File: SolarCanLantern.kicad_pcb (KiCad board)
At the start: 2 copper layers, 30.5 x 19 mm, 15 parts, among them Q1 2N7002, Q2 2N7002, SW1 SW_Push, U1 ATTINY13-20SSU, U2 MAX40200

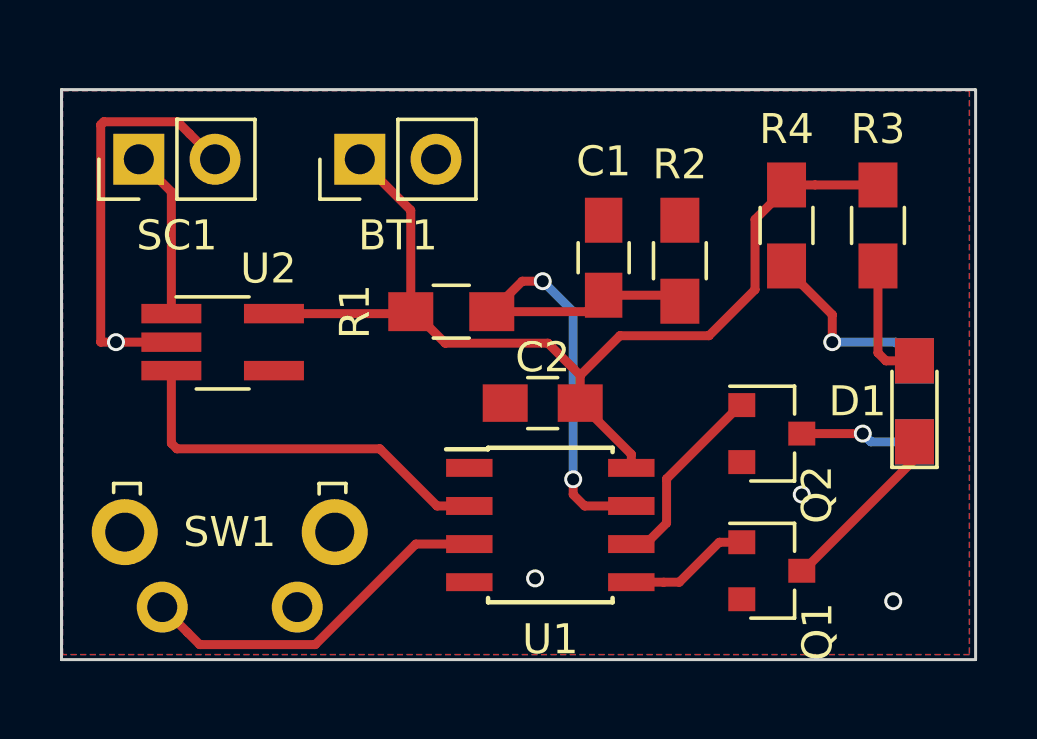
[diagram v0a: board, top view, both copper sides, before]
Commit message: slightly reorganize board
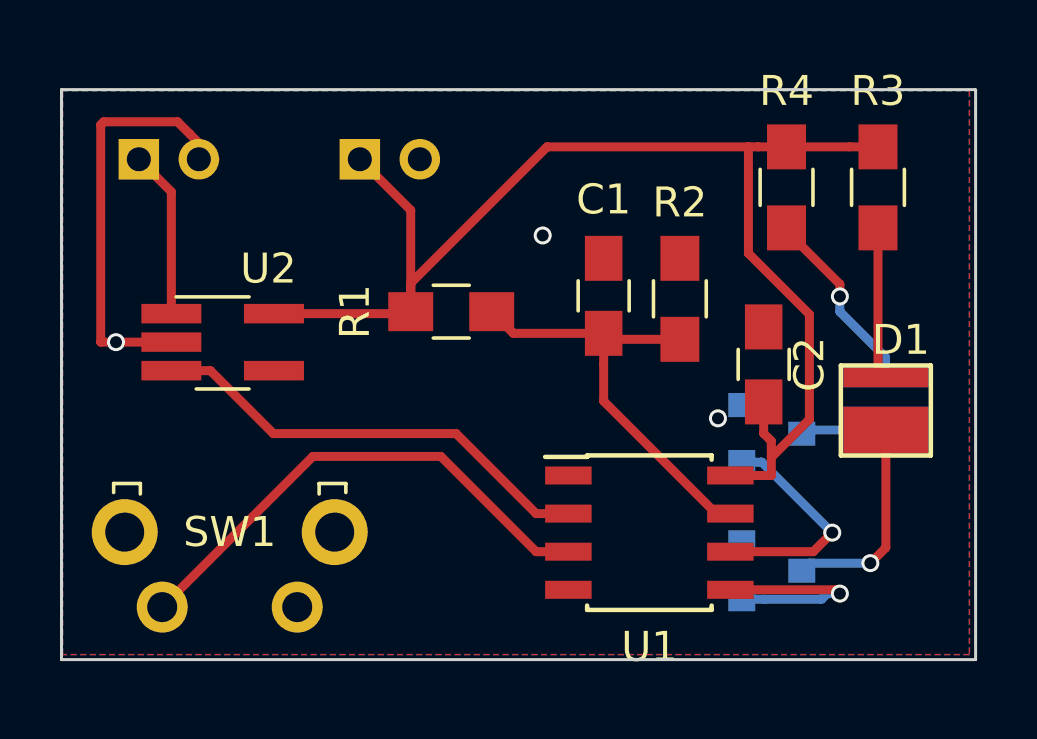
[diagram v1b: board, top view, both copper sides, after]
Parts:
- BT1, SC1: footprint Socket_Strips:Socket_Strip_Straight_1x02_Pitch2.54mm -> Socket_Strips:Socket_Strip_Straight_1x02_Pitch2.00mm; moved to B.Cu
- D1, D2: footprint LEDs:LED_0805_HandSoldering -> Footprints:CreeXLampXH-G
- Q1, Q2: moved to B.Cu
- moved C2 7.48 mm to (220.5, 87.1), turned to 90 degrees
- moved U1 3.31 mm to (216.7, 92.7)
- moved D2 1.48 mm to (224.0, 88.1)
- moved C1 1.27 mm to (215.1, 84.8)
- moved R2 1.27 mm to (217.7, 84.9)
- moved R3 1.27 mm to (224.3, 81.2)
- moved R4 1.27 mm to (221.2, 81.2)
- moved D1 0.49 mm to (225.0, 88.1)
- turned BT1 to 270 degrees
- turned SC1 to 270 degrees
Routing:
- net +BATT: track 34.7 -> 44.6 mm
- net /Switch: track 12.1 -> 16.9 mm
- net /VBatt_Divider: track 18.3 -> 14.7 mm, vias 2 -> 0
- net /LEDA: track 4.23 -> 7.05 mm, vias 0 -> 1
- net /~SOLAR: track 13.2 -> 15.2 mm
- net /LEDB: track 6.47 -> 7.65 mm, vias 0 -> 1
- net Net-(D1-Pad1): track 5.88 -> 7.04 mm, vias 0 -> 1
- net Net-(D2-Pad1): track 3.87 -> 2.84 mm, vias 1 -> 0
- net Net-(D1-Pad2): track 4.22 -> 5.10 mm
- net GND: vias 4 -> 3
